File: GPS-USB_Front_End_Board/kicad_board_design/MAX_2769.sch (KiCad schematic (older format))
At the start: 47 parts, among them J2 Edge Launch SMA, J3 Edge Launch SMA, U4 SAWTEK-855969, U5 AP131-30, U6 MAX2769CETI+, U7 SAWTEK-855969, X1 TCXO3

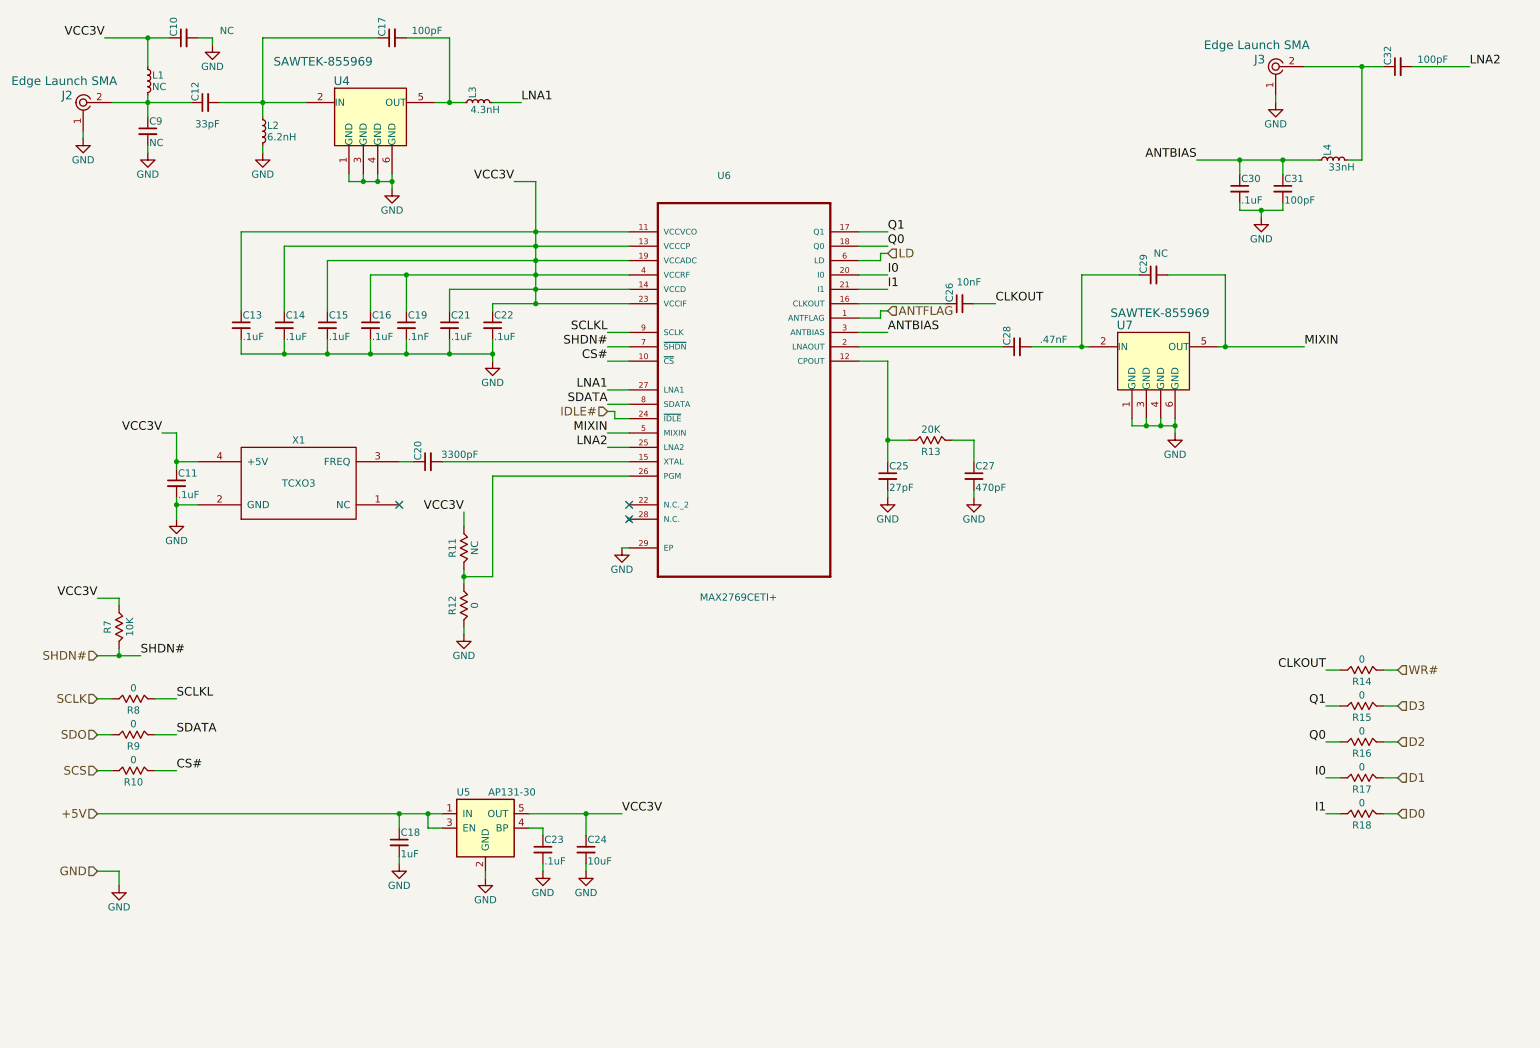
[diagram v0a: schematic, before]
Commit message: Completed, reviewed usb_gps board design.
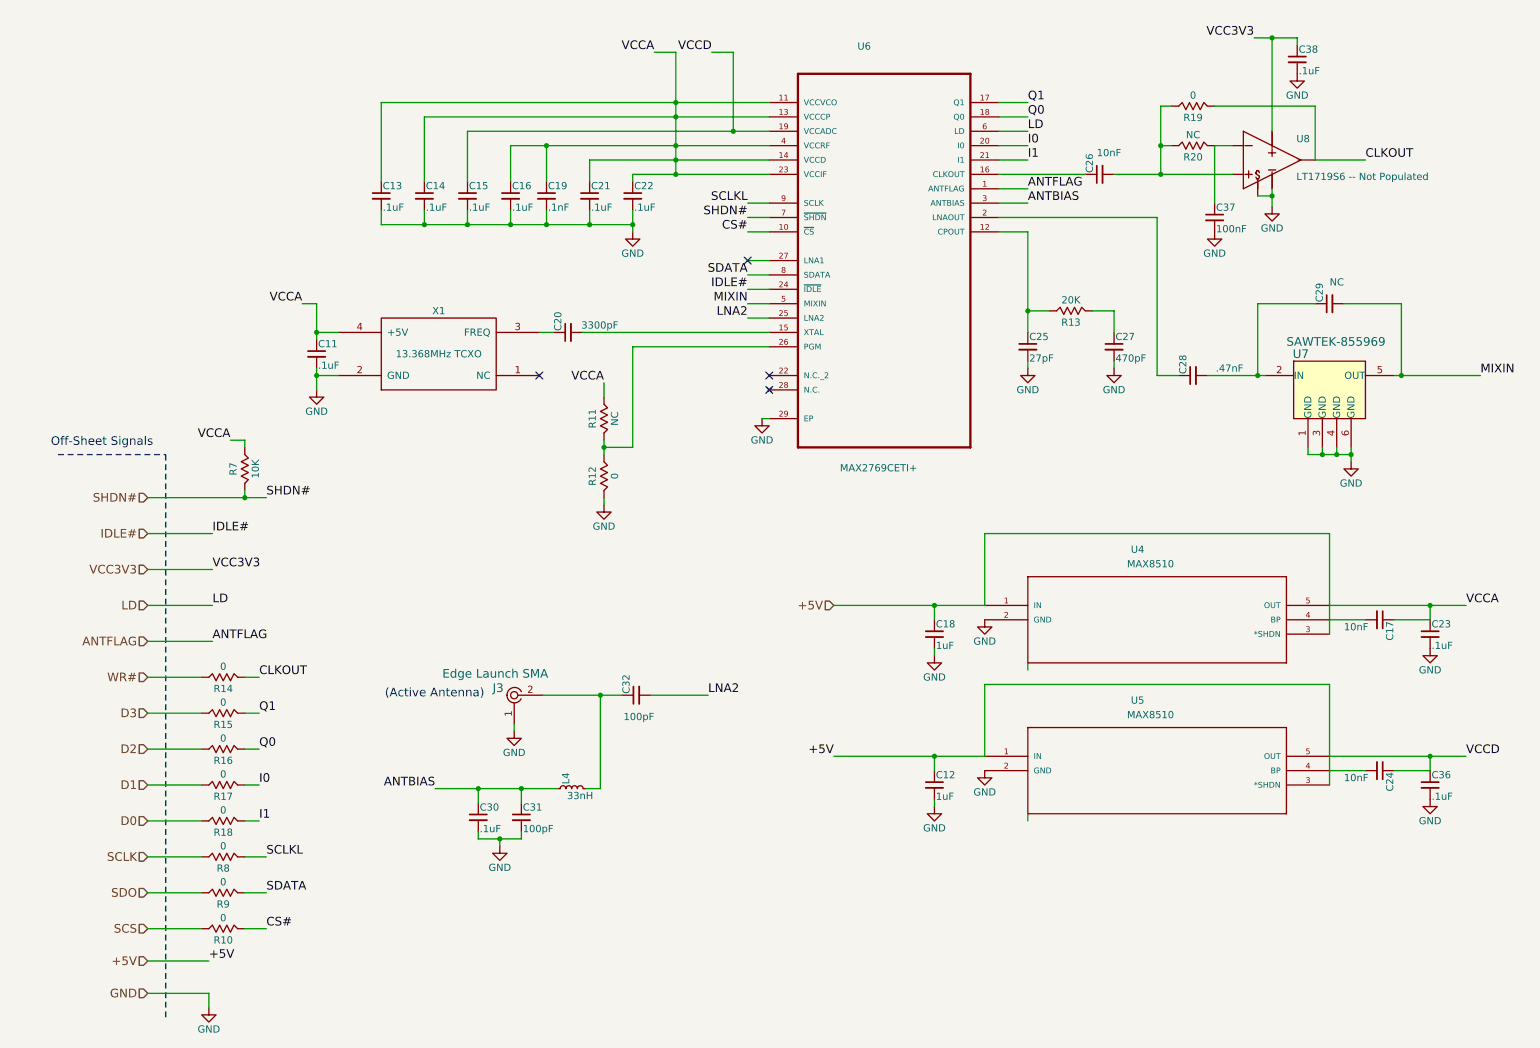
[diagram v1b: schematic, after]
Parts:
- removed C10, C9: NC, Capacitors_SMD:C_0805_HandSoldering, symbol C_Small
- removed J2: Edge Launch SMA, digikey-footprints:RF_SMA_Receptical_Vertical_CONSMA001-SMD-G, symbol CONSMA001-SMD-G
- removed L1: NC, Choke_SMD:Choke_SMD_1206_Handsoldering, symbol L_Small
- removed L2: 6.2nH, Capacitors_SMD:C_0603_HandSoldering, symbol L_Small
- removed L3: 4.3nH, Capacitors_SMD:C_0402, symbol L_Small
- removed U4: SAWTEK-855969, rf:Sawtek_855969, symbol SAWTEK-855969
- removed U5: AP131-30, TO_SOT_Packages_SMD:SOT-23-5, symbol AP131-30
- added C36, C38: .1uF, Capacitors_SMD:C_0402, symbol C_Small
- added C37: 100nF, Capacitors_SMD:C_0402, symbol C_Small
- added R19: 0, Resistors_SMD:R_0603_HandSoldering, symbol R
- added R20: NC, Resistors_SMD:R_0603_HandSoldering, symbol R
- added U4, U5: MAX8510, rf:21-0076E, symbol MAX8510EXK21
- added U8: LT1719S6 -- Not Populated, rf:TSOT-23_S6, symbol LT1719S6
- C12: value 33pF -> 1uF
- C17: value 100pF -> 10nF; footprint Capacitors_SMD:C_0805_HandSoldering -> Capacitors_SMD:C_0402
- C24: value 10uF -> 10nF; footprint Capacitors_SMD:C_0805_HandSoldering -> Capacitors_SMD:C_0402
- X1: value TCXO3 -> 13.368MHz TCXO; footprint oscillator:CTS_405_xtal -> rf:TCXO_Taitien
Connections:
- net +5V: now also C12.1, U4.1 (IN), U4.3 (*SHDN), U5.1 (IN), U5.3 (*SHDN)
- net CLKOUT: now also R14.1, R19.1, U8.5 (OUT); no longer C26.2, R14.2
- net D0: now also R18.2; no longer R18.1
- net D1: now also R17.2; no longer R17.1
- net D2: now also R16.2; no longer R16.1
- net D3: now also R15.2; no longer R15.1
- net GND: now also C12.2, C36.2, C37.2, C38.2, U4.2 (GND), U5.2 (GND), U8.2 (V-), U8.6 (SHDN); no longer C24.2
- net I0: now also R17.1; no longer R17.2
- net I1: now also R18.1; no longer R18.2
- net Q0: now also R16.1; no longer R16.2
- net Q1: now also R15.1; no longer R15.2
- net WR#: now also R14.2; no longer R14.1
- net VCCA: now reaches C17.1
- net VCCA: now also C11.1, C13.1, C14.1, C16.1, C19.1, C21.1, C22.1, C23.1, R11.2, R7.2, U6.11 (VCCVCO), U6.13 (VCCCP), U6.14 (VCCD), U6.23 (VCCIF), U6.4 (VCCRF), X1.4 (+5V), U4.5 (OUT); no longer C12.2
- net at C17.2: now also U4.4 (BP)
- net LNA1: no longer names the net of U6.27 (LNA1)
- removed net VCC3V: C11.1, C13.1, C14.1, C15.1, C16.1, C19.1, C21.1, C22.1, C24.1, R11.2, R7.2, U6.11 (VCCVCO), U6.13 (VCCCP), U6.14 (VCCD), U6.19 (VCCADC), U6.23 (VCCIF), U6.4 (VCCRF), X1.4 (+5V)
- new net: C26.2, R19.2, R20.2, U8.3 (IN+)
- new net: C24.2, U5.4 (BP)
- new net: C37.1, R20.1, U8.1 (IN)
- new net VCC3V3: C38.1, U8.4 (V+)
- new net VCCD: C15.1, C24.1, C36.1, U5.5 (OUT), U6.19 (VCCADC)
- no-connect marks 3 -> 4
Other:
- note added: "(Active Antenna)"
- note added: "Off-Sheet Signals"
- moved on the sheet: C11, C13, C14, C15, C16, C18, C19, C20, C21, C22, C23, C25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

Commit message: schematic cleanup
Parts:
- C11, C13, C14, C15, C16, C21, C22, C23, C30, C36, C37, C38: MFR (none) -> TDK; MPN (none) -> CGA2B1X7R1C104K050BC; SPN (none) -> 445-5613-1-ND; SPR (none) -> Digikey; SPURL (none) -> -
- C12, C18: MFR (none) -> Samsung; MPN (none) -> CL10B105KP8NNNC; SPN (none) -> 1276-1946-1-ND; SPR (none) -> Digikey; SPURL (none) -> -
- C17, C24, C26: MFR (none) -> Murata; MPN (none) -> GRM155R71C103KA01D; SPN (none) -> 490-1313-1-ND; SPR (none) -> Digikey; SPURL (none) -> -
- C19, C31, C32: MFR (none) -> Kemet; MPN (none) -> C0805C101K4RAC7800; SPN (none) -> 399-15003-1-ND; SPR (none) -> Digikey; SPURL (none) -> -
- C20: MFR (none) -> AVX; MPN (none) -> 06035C332KAT4A; SPN (none) -> 478-10681-1-ND; SPR (none) -> Digikey; SPURL (none) -> -
- C25: MFR (none) -> AVX; MPN (none) -> 08055C270KAT2A; SPN (none) -> 478-11394-1-ND; SPR (none) -> Digikey; SPURL (none) -> -
- C27, C28: MFR (none) -> AVX; MPN (none) -> 04025C471KAT2A; SPN (none) -> 478-1097-1-ND; SPR (none) -> Digikey; SPURL (none) -> -
- C29, R10, R11, R12, R14, R15, R16, R17, R18, R19, R20, R8, R9: MFR (none) -> Vishay; MPN (none) -> CRCW06030000Z0EBC; SPN (none) -> 541-4013-1-ND; SPR (none) -> Digikey; SPURL (none) -> -
- J3: MFR (none) -> Linx Technologies; SPN (none) -> CONSMA001-SMD-G-ND; SPR (none) -> Digikey; SPURL (none) -> -
- L4: MFR (none) -> Bourns; MPN (none) -> CI100505-33NJ; SPN (none) -> CI100505-33NJCT-ND; SPR (none) -> Digikey; SPURL (none) -> -
- R13: MFR (none) -> Bourns; MPN (none) -> CRT0603-FZ-2002EST; SPN (none) -> CRT0603-FZ-2002ESTCT-ND; SPR (none) -> Digikey; SPURL (none) -> -
- R7: MFR (none) -> TE Connectivity; MPN (none) -> CRGH0805F10K; SPN (none) -> A126417DKR-ND; SPR (none) -> Digikey; SPURL (none) -> -
- U4, U5: MFR (none) -> Maxim; MPN (none) -> MAX8510EXK30+T; SPN (none) -> MAX8510EXK30+TCT-ND; SPR (none) -> Digikey; SPURL (none) -> -
- U6: MFR (none) -> Maxim; MPN (none) -> MAX2769CETI+; SPN (none) -> 700-MAX2769CETI+; SPR (none) -> Mouser; SPURL (none) -> -
- U7: MFR (none) -> Qorvo; MPN AP2114H-3.3TRG1 -> 855969; SPN (none) -> 772-855969; SPR (none) -> Mouser; SPURL (none) -> -
- U8: MFR (none) -> Linear Tech; MPN (none) -> LT1719IS6#TRMPBF; SPN (none) -> LT1719IS6#TRMPBFCT-ND; SPR (none) -> Digikey; SPURL (none) -> -
- X1: MFR (none) -> Taitien; MPN (none) -> TXETCDSANF-16.368000; SPN (none) -> 1664-1271-1-ND; SPR (none) -> Digikey; SPURL (none) -> -
